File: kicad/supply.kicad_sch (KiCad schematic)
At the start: 38 parts, among them J5 Screw_Terminal_01x03, U14 TMUX6123, U15 TMUX6123, U6 LM2937-5, U9 LM317_TO-252

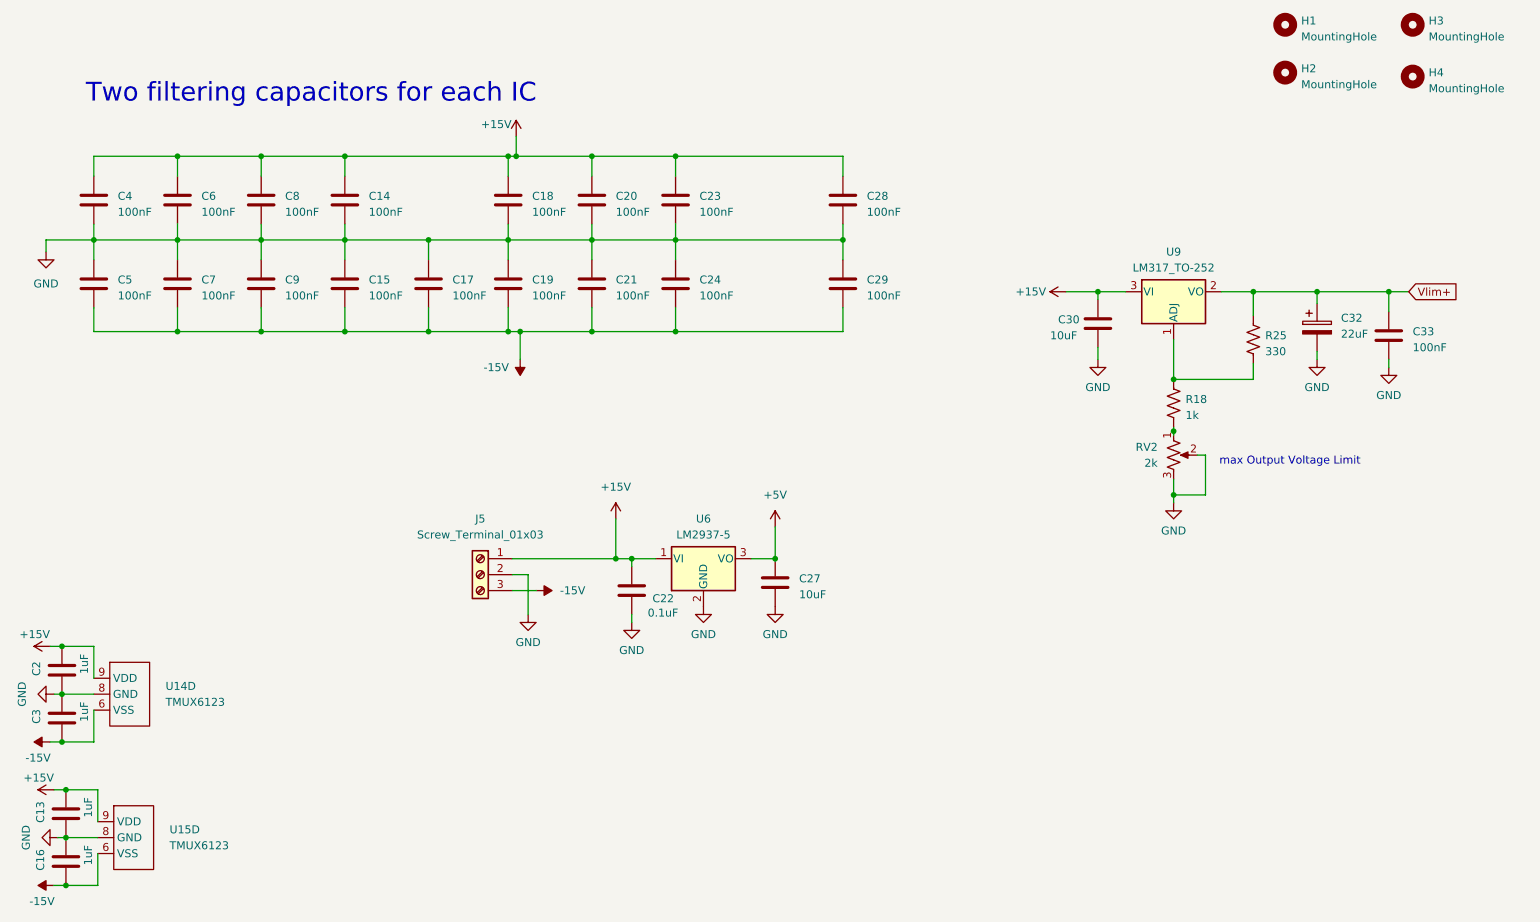
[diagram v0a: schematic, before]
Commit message: First portion of routing
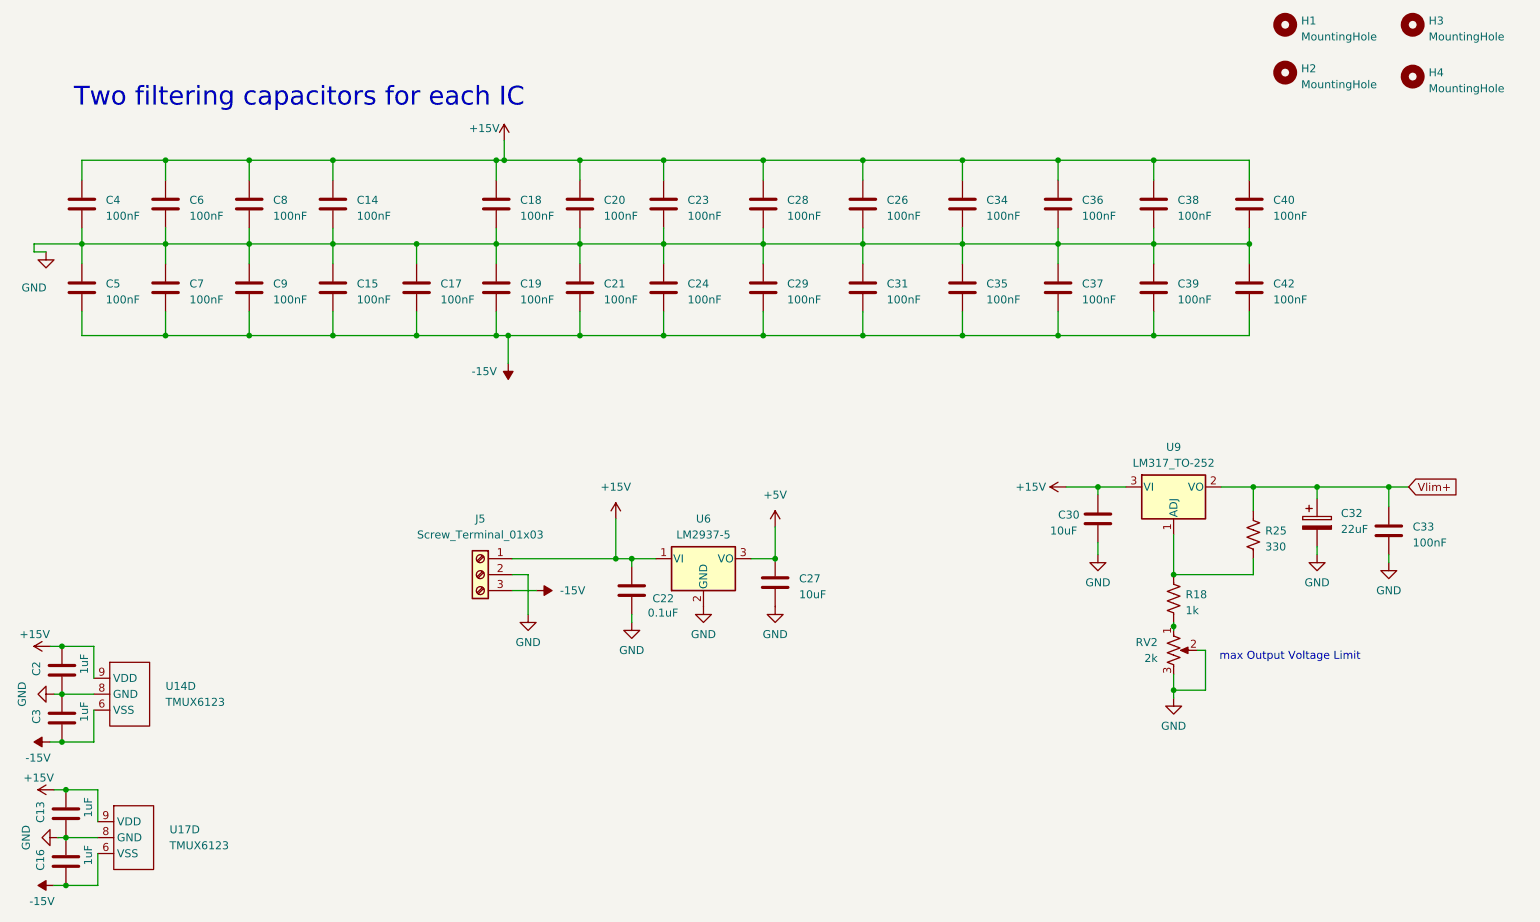
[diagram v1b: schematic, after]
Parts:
- added C26, C31, C34, C35, C36, C37, C38, C39, C40, C42: 100nF, Capacitor_SMD:C_0805_2012Metric, symbol Device:C
- renumbered U15 to U17
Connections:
- net +15V: now also C26.1, C34.1, C36.1, C38.1, C40.1
- net -15V: now also C31.2, C35.2, C37.2, C39.2, C42.2
- net GND: now also C26.2, C31.1, C34.2, C35.1, C36.2, C37.1, C38.2, C39.1, C40.2, C42.1
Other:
- moved on the sheet: C14, C15, C17, C18, C19, C20, C21, C23, C24, C28, C29, C30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
